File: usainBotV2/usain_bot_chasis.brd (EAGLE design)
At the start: 100 x 80 mm, 10 parts, among them X1 22-23-2021, X2 22-23-2021, X3 22-23-2021

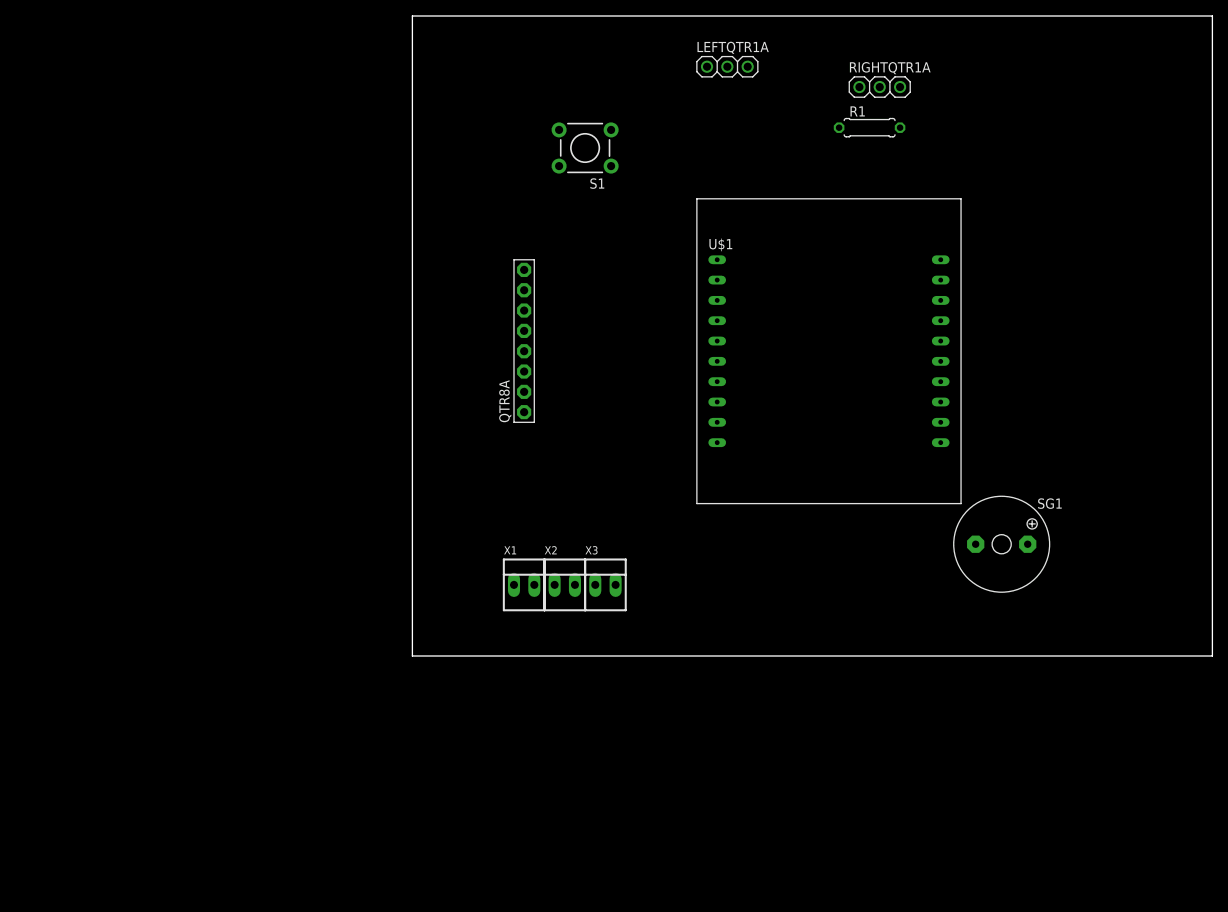
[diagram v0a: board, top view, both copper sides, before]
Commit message: carpetas ordenadas y limpias, proyectos de pcbs en este repo
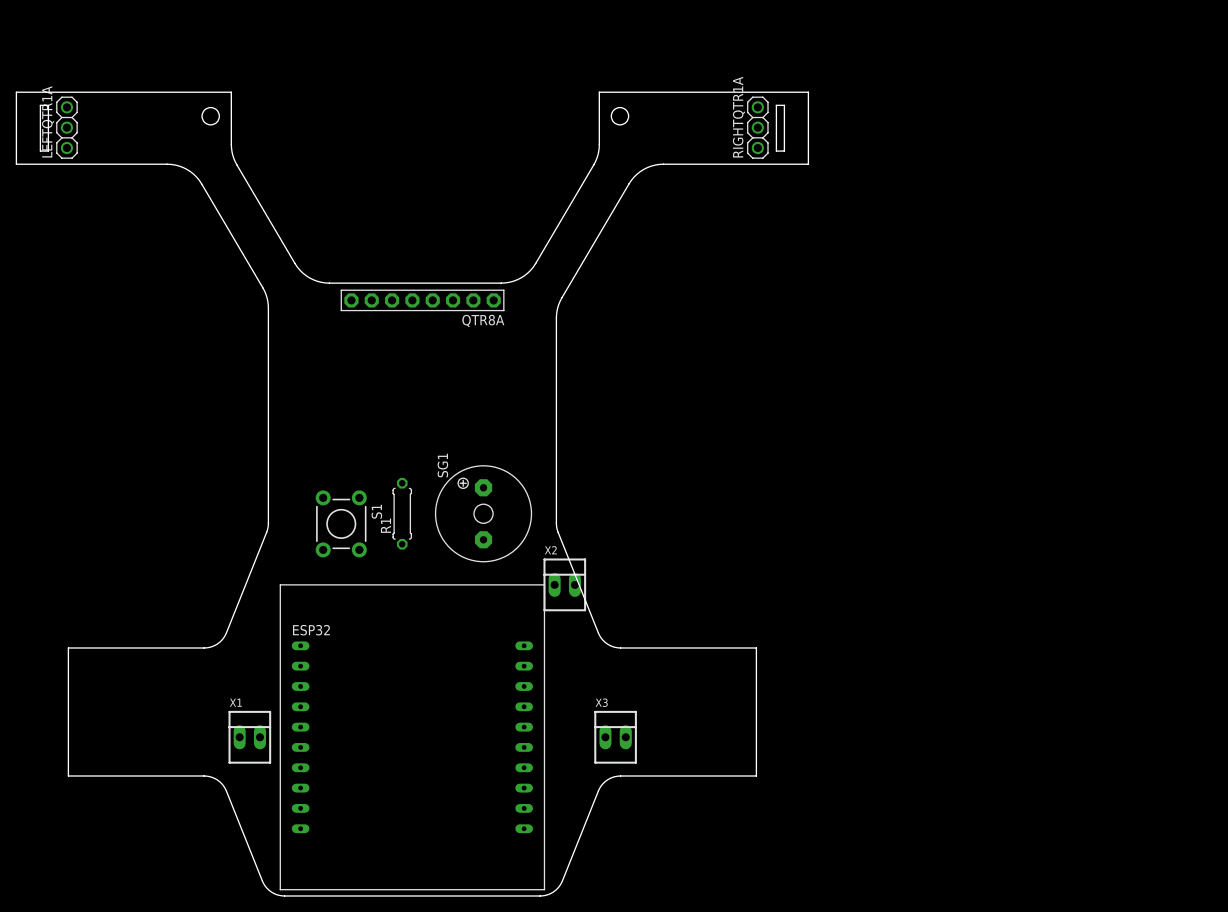
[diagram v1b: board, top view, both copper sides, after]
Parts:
- removed U$1: ESP32_MINI_KIT, dedo:ESP32_MINI_KIT
- added ESP32: ESP32_MINI_KIT, dedo:ESP32_MINI_KIT
- moved LEFTQTR1A 82.9 mm to (-43.2, 66.0), turned to 90 degrees
- moved R1 75.8 mm to (-1.27, 17.8), turned to 90 degrees
- moved SG1 64.9 mm to (8.89, 17.8), turned to 90 degrees
- moved S1 56.0 mm to (-8.89, 16.5), turned to 270 degrees
- moved X1 39.2 mm to (-20.3, -10.2)
- moved X3 19.1 mm to (25.4, -10.2)
- moved RIGHTQTR1A 16.1 mm to (43.2, 66.0), turned to 90 degrees
- moved QTR8A 13.7 mm to (1.27, 44.5), turned to 180 degrees
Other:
- board size 100 x 80 mm -> 99 x 100.5 mm
